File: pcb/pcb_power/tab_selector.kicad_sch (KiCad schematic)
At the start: 2 parts, among them K1 FINDER-40.41, K2 FINDER-40.41

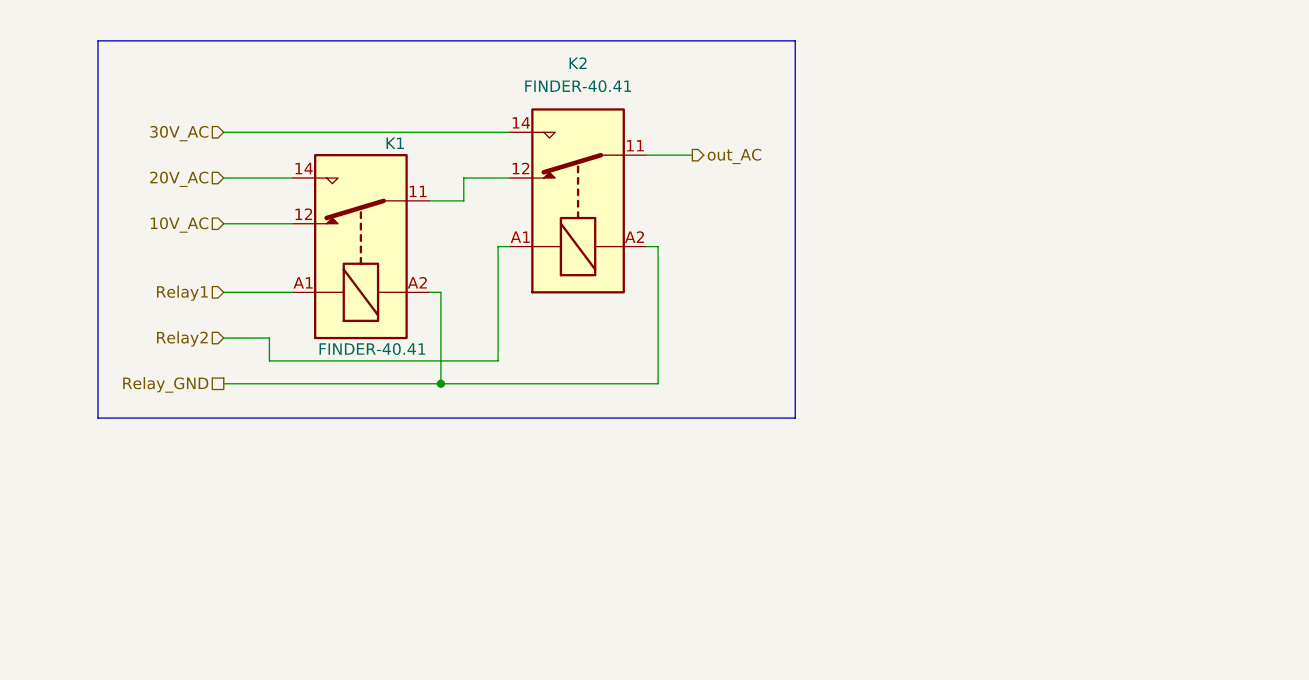
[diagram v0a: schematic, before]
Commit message: fin board
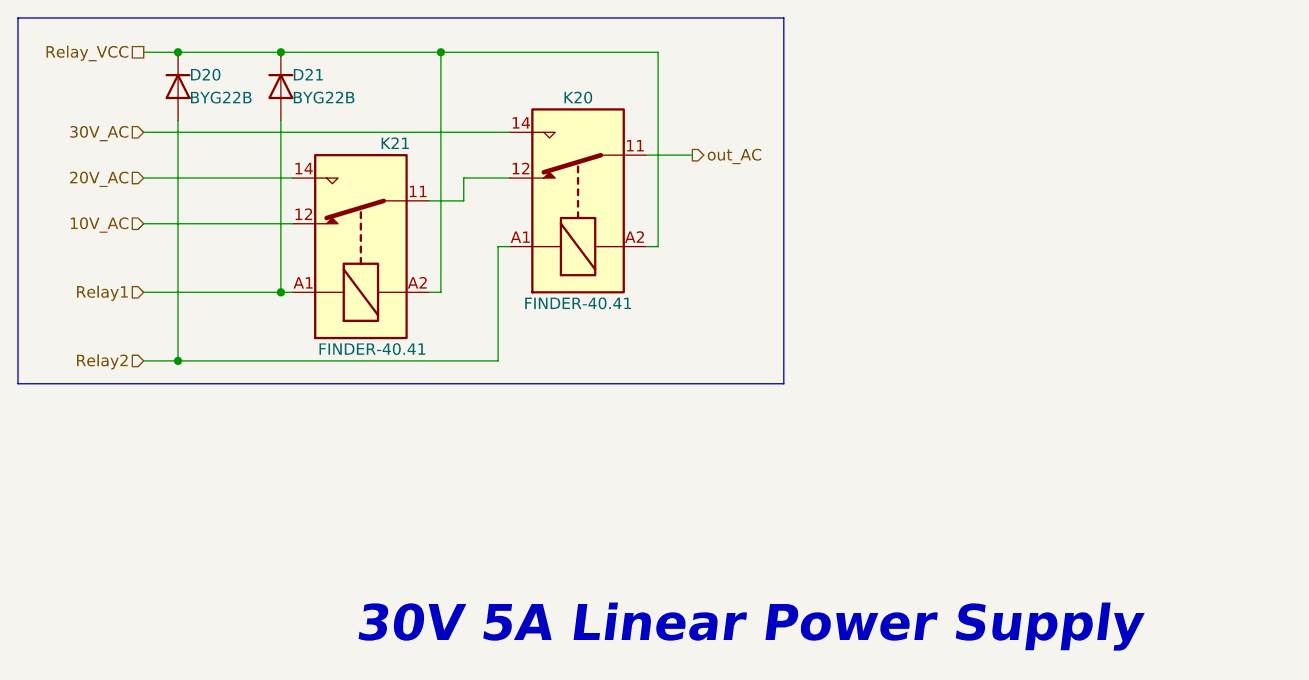
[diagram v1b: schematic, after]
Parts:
- added D20, D21: BYG22B, Diode_SMD:D_SMA, symbol Diode:1N4148WT
- renumbered K2 to K20, K1 to K21
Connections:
- net Relay1: now also D21.2 (A)
- net Relay2: now also D20.2 (A)
- net Relay_GND renamed Relay_VCC
- net Relay_VCC: now also D20.1 (K), D21.1 (K)
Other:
- note added: "30V 5A Linear Power Supply"
